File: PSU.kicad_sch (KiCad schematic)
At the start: 10 parts, among them J1 Mini USB Female, J4 Battery Connector, SW1 Screw Switch, U2 AMS1117-3.3

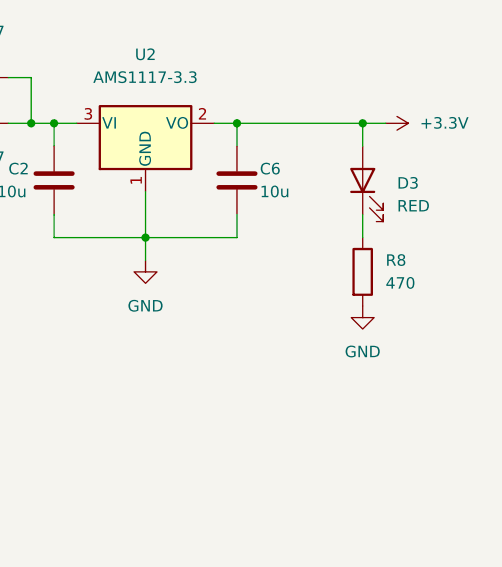
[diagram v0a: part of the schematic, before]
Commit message: Experimented with git
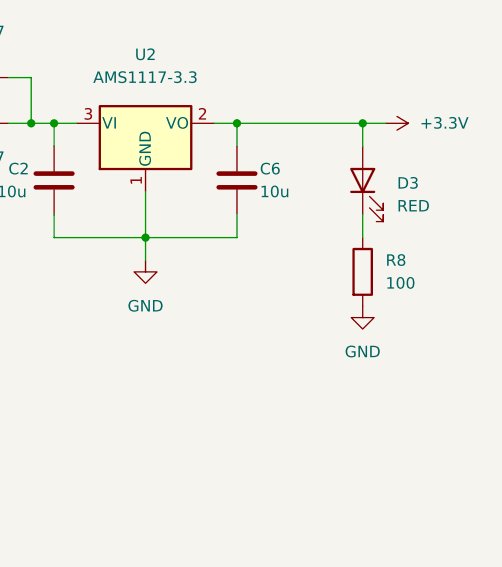
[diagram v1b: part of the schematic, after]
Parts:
- R8: value 470 -> 100
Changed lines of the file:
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@@
       (effects (font (size 1.27 1.27)) (justify left))
     )
-    (property "Value" "470" (id 1) (at 177.8 82.5499 0)
+    (property "Value" "100" (id 1) (at 177.8 82.5499 0)
       (effects (font (size 1.27 1.27)) (justify left))
     )
